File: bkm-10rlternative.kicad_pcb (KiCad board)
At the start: 4 copper layers, 210.8 x 74.9 mm, 257 parts, among them J1 DB9_Male_MountingHoles, J2 ICSP, Q1 MMBT3904, Q10 MMBT3904, Q11 MMBT3904, Q12 MMBT3904, Q13 MMBT3904, Q14 MMBT3904, Q2 MMBT3904, Q3 MMBT3904, Q4 MMBT3904, Q5 MMBT3904, Q6 MMBT3904, Q7 MMBT3904, Q8 MMBT3904, Q9 MMBT3904, SW1 SHIFT, SW10 ADDR_SAFE_AREA, SW11 UP, SW12 MENU, SW13 DOWN, SW14 ENTER, SW15 DEGAUSS, SW16 POWER, SW17 KEY_1, SW18 KEY_2, SW19 KEY_3, SW2 HORIZ_SYNC, SW20 KEY_4, SW21 KEY_5, SW22 KEY_6, SW23 KEY_7, SW24 KEY_8, SW25 KEY_9, SW26 KEY_DEL, SW27 KEY_0, SW28 KEY_ENTER, SW29 CONTRAST_MANUAL, SW3 UNDERSCAN_16_9, SW30 CONTRAST_KNOB, SW31 BRIGHT_MANUAL, SW32 BRIGHT_KNOB, SW33 CHROMA_MANUAL, SW34 CHROMA_KNOB, SW35 PHASE_MANUAL, SW36 PHASE_KNOB, SW4 VERT_BLUE_ONLY, SW5 MONO_R, SW6 APT_G, SW7 COMB_B, SW8 F1_F3, SW9 F2_F4, U1 74LVC2G14, U10 MCP23S17_SS, U11 MCP23S17_SS, U12 MCP23S17_SS, U13 74LVC2G14, U14 74LVC2G14, U15 74LVC2G14, U16 74LVC2G14, U17 74LVC2G14, U18 74LVC2G14, U19 74LVC2G14, U2 74HC14, U20 74LVC2G14, U3 74HC14, U4 74HC14, U5 74HC14, U6 TSOP382xx, U8 MAX491E, U9 ATmega328PB-AU, Y1 Resonator

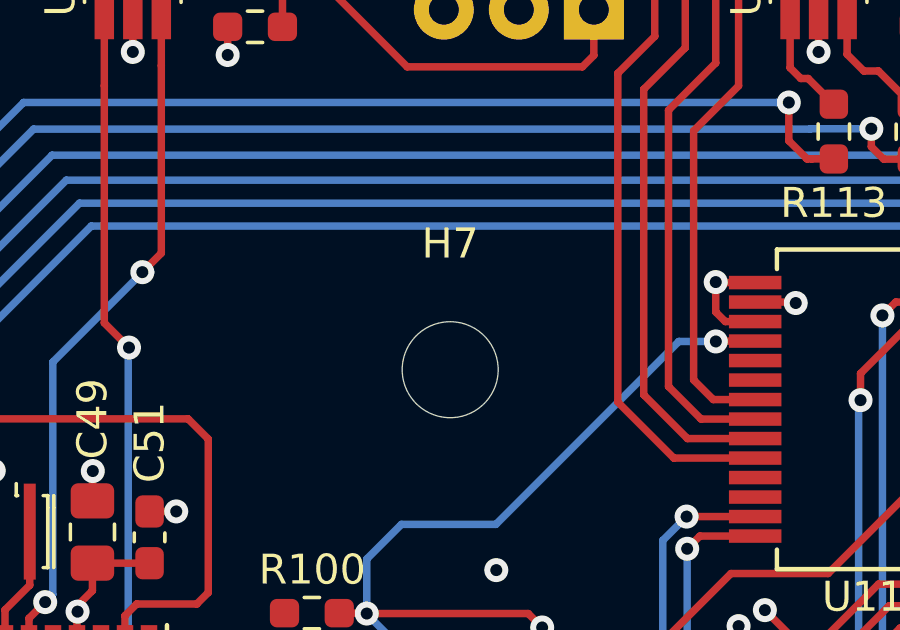
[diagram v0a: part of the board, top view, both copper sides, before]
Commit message: 3D files and minor stuff
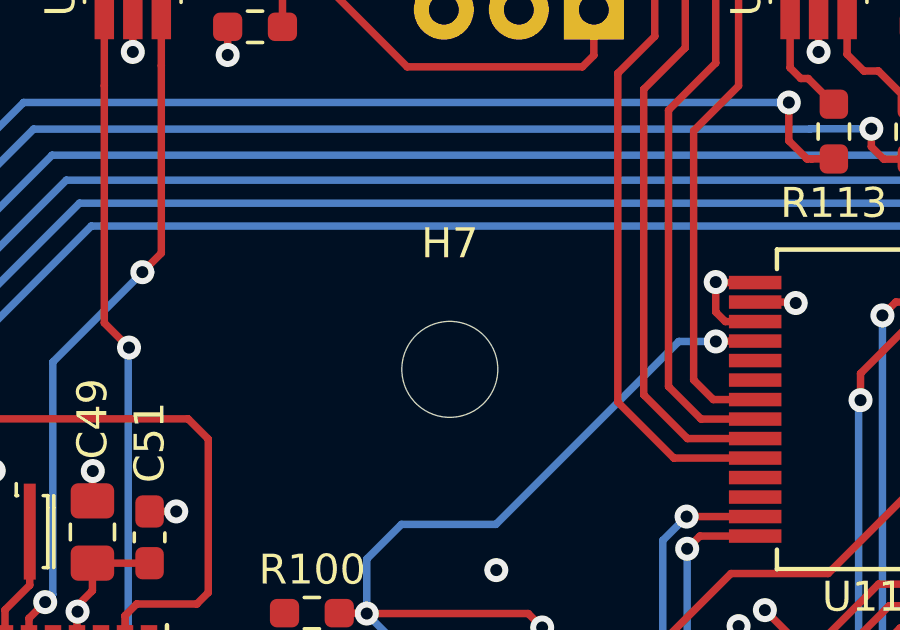
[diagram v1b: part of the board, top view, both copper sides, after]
